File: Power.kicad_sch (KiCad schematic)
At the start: 28 parts, among them J1 12V, J11 Conn_01x02_Pin, J14 Conn_01x02_Pin, J15 Conn_01x02_Pin, U1 TPS7A2633DRVR, U2 TPS54202DDC

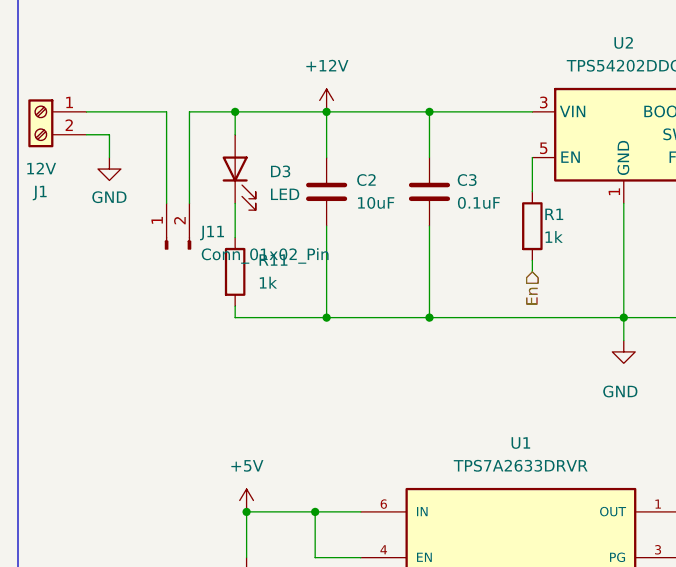
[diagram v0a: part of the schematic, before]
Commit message: Update schemtic
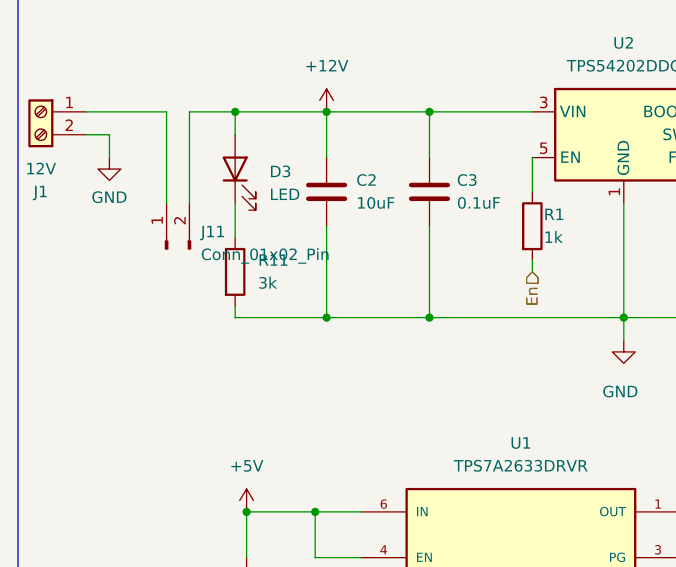
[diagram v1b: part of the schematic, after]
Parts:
- R11: value 1k -> 3k
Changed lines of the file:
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@@
 			)
 		)
-		(property "Value" "1k"
+		(property "Value" "3k"
 			(at 101.6 85.0899 0)
 			(effects
